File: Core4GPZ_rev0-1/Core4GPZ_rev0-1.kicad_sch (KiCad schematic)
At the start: 12 parts, among them U2 core4, U3 MPXHZ6250AC6T1, U5 LMV321

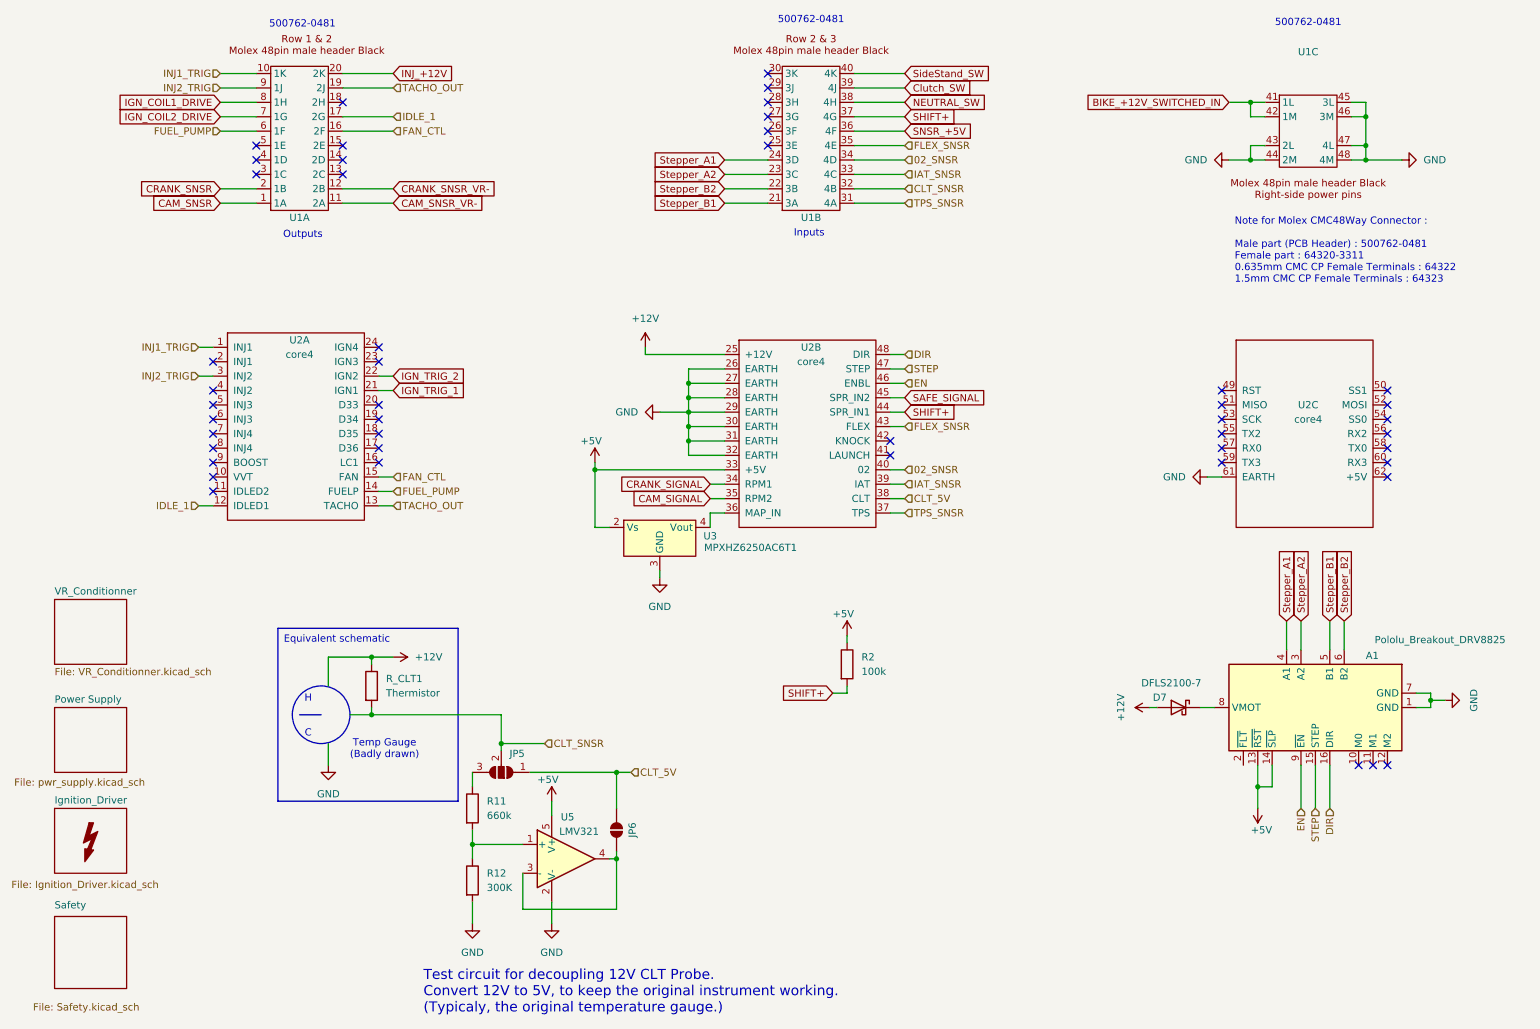
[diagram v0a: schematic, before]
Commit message: Reorganised Schematic
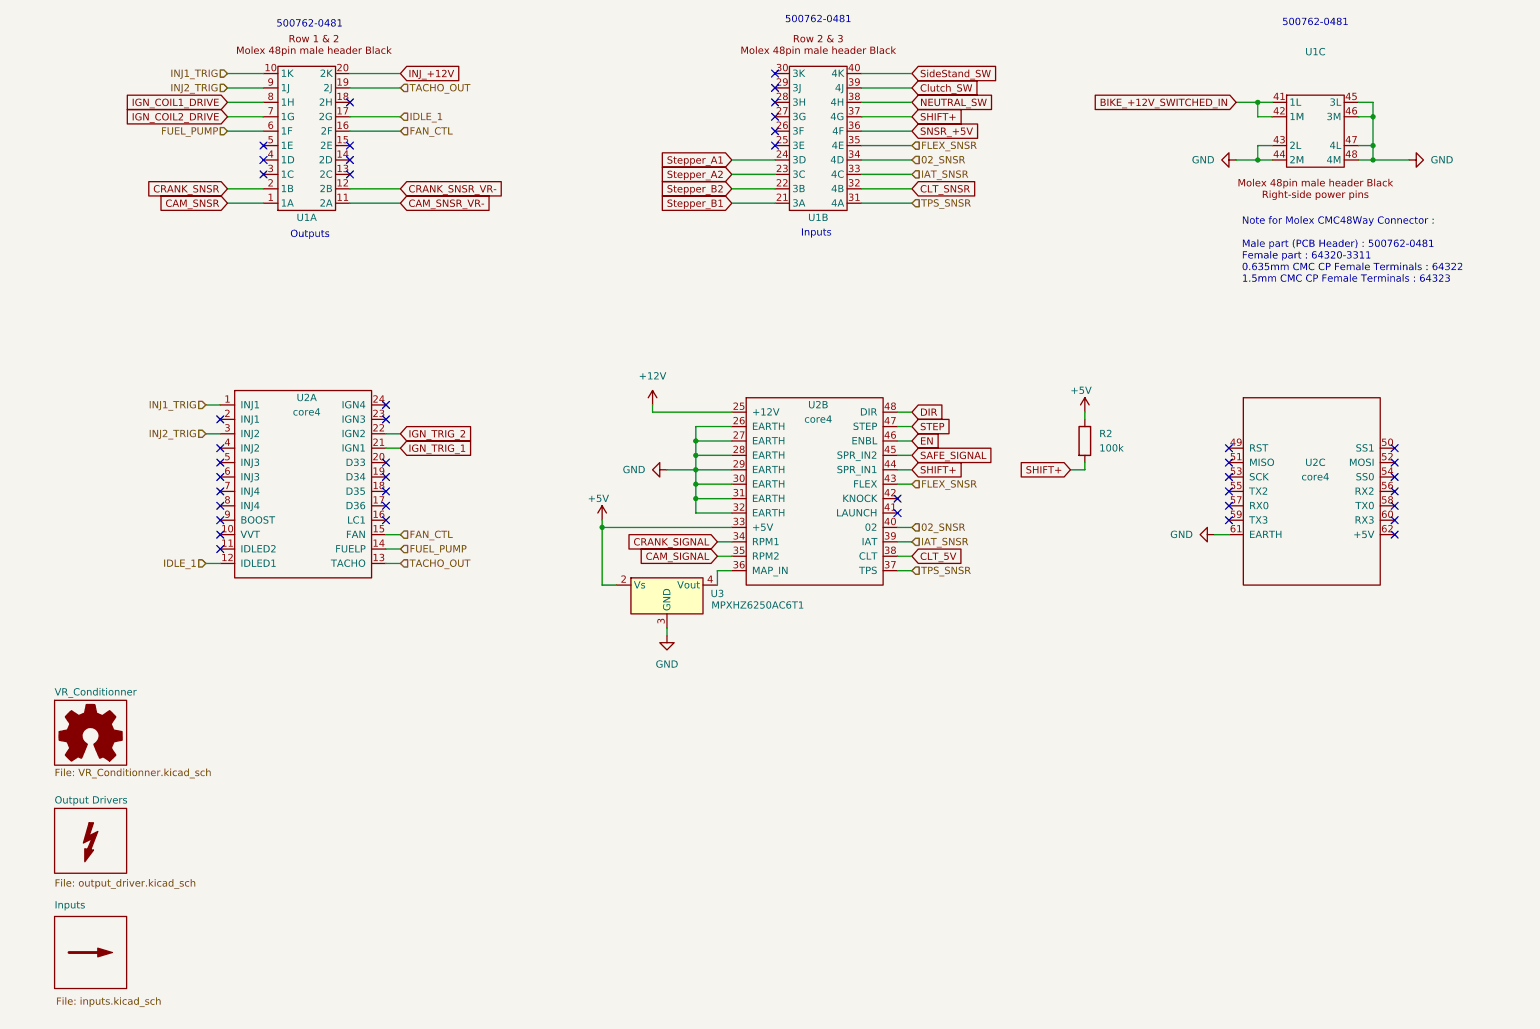
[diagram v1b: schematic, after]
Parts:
- removed A1: Pololu_Breakout_DRV8825, Module:Pololu_Breakout-16_15.2x20.3mm, symbol Driver_Motor:Pololu_Breakout_DRV8825
- removed D7: D_Schottky, Diode_SMD:D_PowerDI-123, symbol Device:D_Schottky
- removed JP5: SolderJumper_3_Open, Jumper:SolderJumper-3_P1.3mm_Open_RoundedPad1.0x1.5mm, symbol Jumper:SolderJumper_3_Open
- removed JP6: SolderJumper_2_Open, Jumper:SolderJumper-2_P1.3mm_Open_RoundedPad1.0x1.5mm, symbol Jumper:SolderJumper_2_Open
- removed R11: 660k, Resistor_SMD:R_0805_2012Metric_Pad1.20x1.40mm_HandSolder, symbol Device:R
- removed R12: 300K, Resistor_SMD:R_0805_2012Metric_Pad1.20x1.40mm_HandSolder, symbol Device:R
- removed R_CLT1: Thermistor, symbol Device:R
- removed U5: LMV321, Package_TO_SOT_SMD:SOT-23-5_HandSoldering, symbol Amplifier_Operational:LMV321
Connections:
- no-connect marks 47 -> 44
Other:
- sheet Ignition_Driver renamed Output Drivers
- sheet Safety renamed Inputs
- removed sheet Power Supply
- sheet Inputs: file Safety.kicad_sch -> inputs.kicad_sch
- sheet Output Drivers: file Ignition_Driver.kicad_sch -> output_driver.kicad_sch
- note removed: "H C"
- note removed: "Temp Gauge (Badly drawn)"
- note removed: "Test circuit for decoupling 12V CLT Probe. Convert 12V to 5V, to keep the original instrument working. (Typicaly, the original temperature gauge.)"
- moved on the sheet: R2, U1A, U1B, U1C, U2A, U2B, U2C, U3
